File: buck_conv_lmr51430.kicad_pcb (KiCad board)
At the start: 2 copper layers, 44.2 x 19.8 mm, 11 parts, among them J1 Screw_Terminal_01x02, J2 Screw_Terminal_01x02

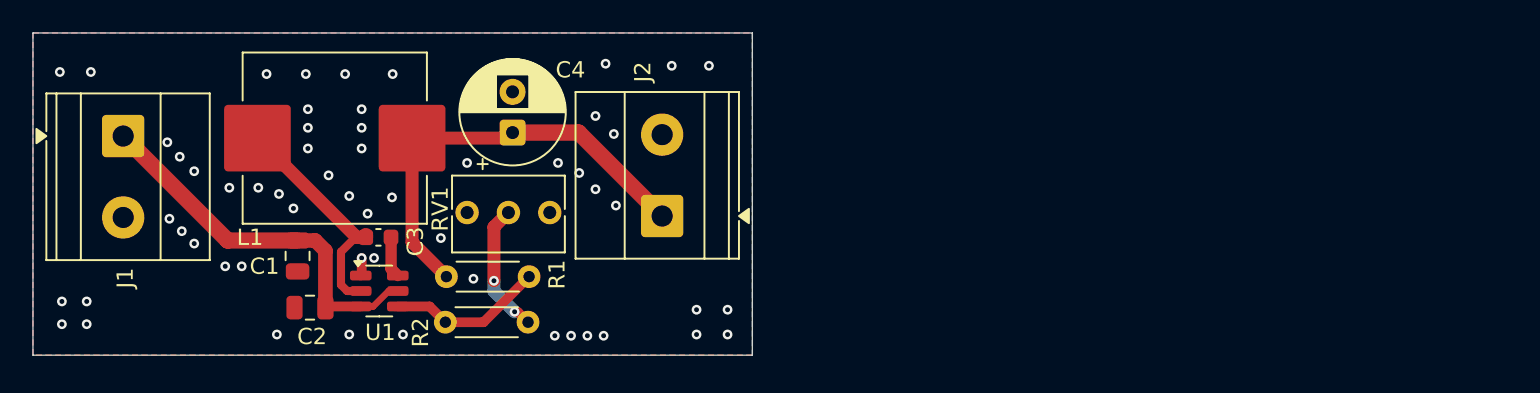
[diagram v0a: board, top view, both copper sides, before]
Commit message: rajath final touches
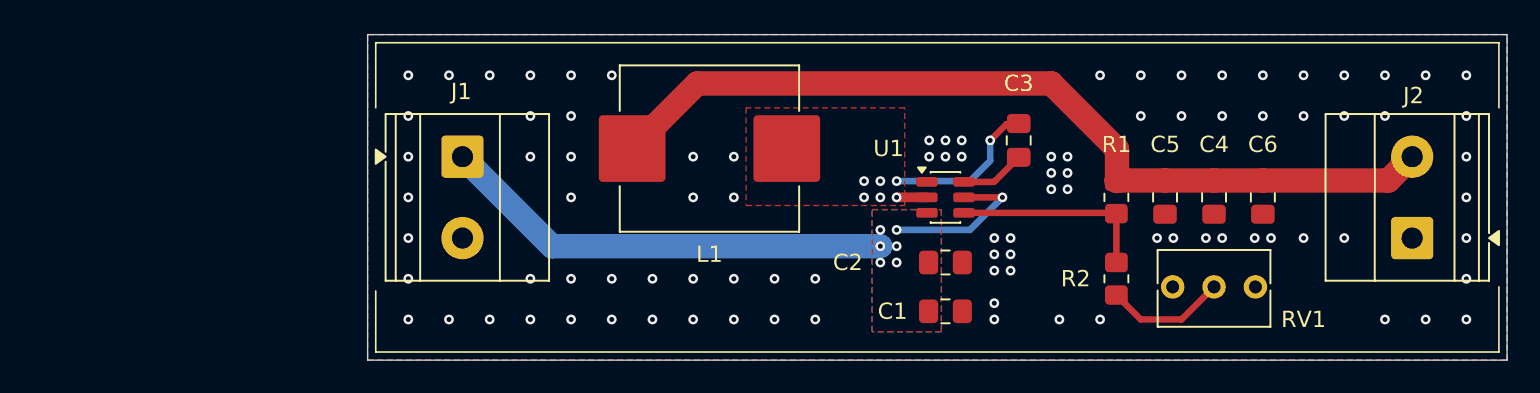
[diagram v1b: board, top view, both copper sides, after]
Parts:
- added C5: 22u, Capacitor_SMD:C_0805_2012Metric_Pad1.18x1.45mm_HandSolder, F.Cu at (169.0, 90.0)
- added C6: 22u, Capacitor_SMD:C_0805_2012Metric_Pad1.18x1.45mm_HandSolder, F.Cu at (175.0, 90.0)
- C1: value 1uF -> 4.7u; footprint Capacitor_SMD:C_0805_2012Metric -> Capacitor_SMD:C_0805_2012Metric_Pad1.18x1.45mm_HandSolder
- C2: value 100nF -> 100n; footprint Capacitor_SMD:C_0805_2012Metric -> Capacitor_SMD:C_0805_2012Metric_Pad1.18x1.45mm_HandSolder
- C3: value 100nF -> 100n; footprint Capacitor_SMD:C_0603_1608Metric -> Capacitor_SMD:C_0805_2012Metric_Pad1.18x1.45mm_HandSolder
- C4: value 100uF -> 22u; footprint Capacitor_THT:CP_Radial_D6.3mm_P2.50mm -> Capacitor_SMD:C_0805_2012Metric_Pad1.18x1.45mm_HandSolder
- J1: value Screw_Terminal_01x02 -> Input
- J2: value Screw_Terminal_01x02 -> Output
- L1: value 5.6uH -> 12u
- R1: value 100k -> 100K; footprint Resistor_THT:R_Axial_DIN0204_L3.6mm_D1.6mm_P5.08mm_Horizontal -> Resistor_SMD:R_0805_2012Metric_Pad1.20x1.40mm_HandSolder
- R2: value 22.1 -> 5K; footprint Resistor_THT:R_Axial_DIN0204_L3.6mm_D1.6mm_P5.08mm_Horizontal -> Resistor_SMD:R_0805_2012Metric_Pad1.20x1.40mm_HandSolder
- RV1: value 200k -> 20K
- U1: value ~ -> LMR51430
- moved J2 46.1 mm to (184.2, 92.5)
- moved RV1 43.6 mm to (174.5, 95.5)
- moved C4 43.3 mm to (172.0, 90.0), turned to -90 degrees
- moved R1 41.4 mm to (166.0, 90.0), turned to -90 degrees
- moved R2 41.3 mm to (166.0, 95.0), turned to -90 degrees
- moved C1 39.9 mm to (155.5, 97.0), turned to 0 degrees
- moved C3 39.8 mm to (160.0, 86.5), turned to 90 degrees
- moved C2 39.1 mm to (155.5, 94.0), turned to 0 degrees
- moved U1 35.3 mm to (155.5, 90.0)
- moved L1 23.0 mm to (141.0, 87.0), turned to 180 degrees
- moved J1 20.9 mm to (125.8, 87.5)
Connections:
- net Net-(J1-Pin_1) renamed /VIN
- net Net-(U1-FB) renamed /FB
- net Net-(U1-SW) renamed /SW
- C4 pad 1: Net-(J2-Pin_1) -> /VOUT
- J2 pad 1: Net-(J2-Pin_1) -> GND
- J2 pad 2: GND -> /VOUT
- L1 pad 2: Net-(J2-Pin_1) -> /VOUT
- R1 pad 1: Net-(J2-Pin_1) -> /VOUT
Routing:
- net /VOUT: track 0.00 -> 53.8 mm
- net Net-(J2-Pin_1): track 27.0 -> 0.00 mm
- net /VIN: track 24.0 -> 37.6 mm, vias 0 -> 7
- net /SW: track 14.6 -> 11.6 mm, vias 0 -> 7
- net /FB: track 9.98 -> 12.4 mm
- net Net-(U1-CB): track 2.52 -> 3.99 mm
- net GND: track 1.10 -> 0.00 mm, vias 57 -> 94
- net Net-(R2-Pad2): track 8.08 -> 7.45 mm, vias 2 -> 0
- added copper zone on F.Cu, net /SW
- added copper zone on B.Cu, net /VIN
- added copper zone on F.Cu, net /VIN
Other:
- board size 44.2 x 19.8 mm -> 70 x 20 mm
